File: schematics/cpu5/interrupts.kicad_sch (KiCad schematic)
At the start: 16 parts, among them U83 74LS08, U84 74LS32, U85 74LS32, U86 74LS04, U87 74LS02, U88 74LS02, U89 74LS08, U90 74LS32, U91 74LS541, U92 74LS32

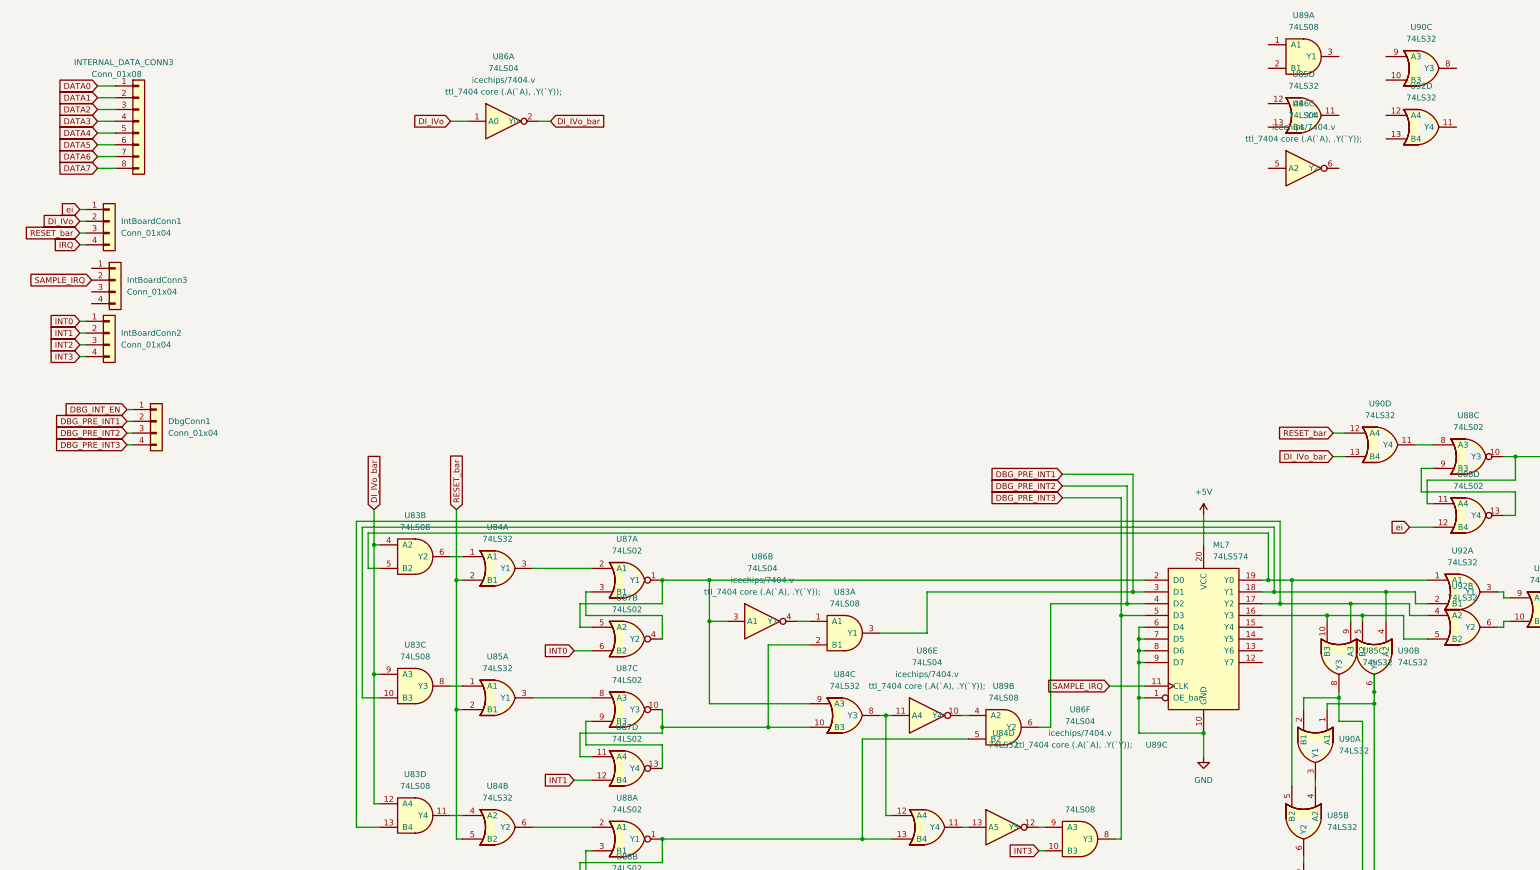
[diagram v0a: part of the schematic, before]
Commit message: start faults
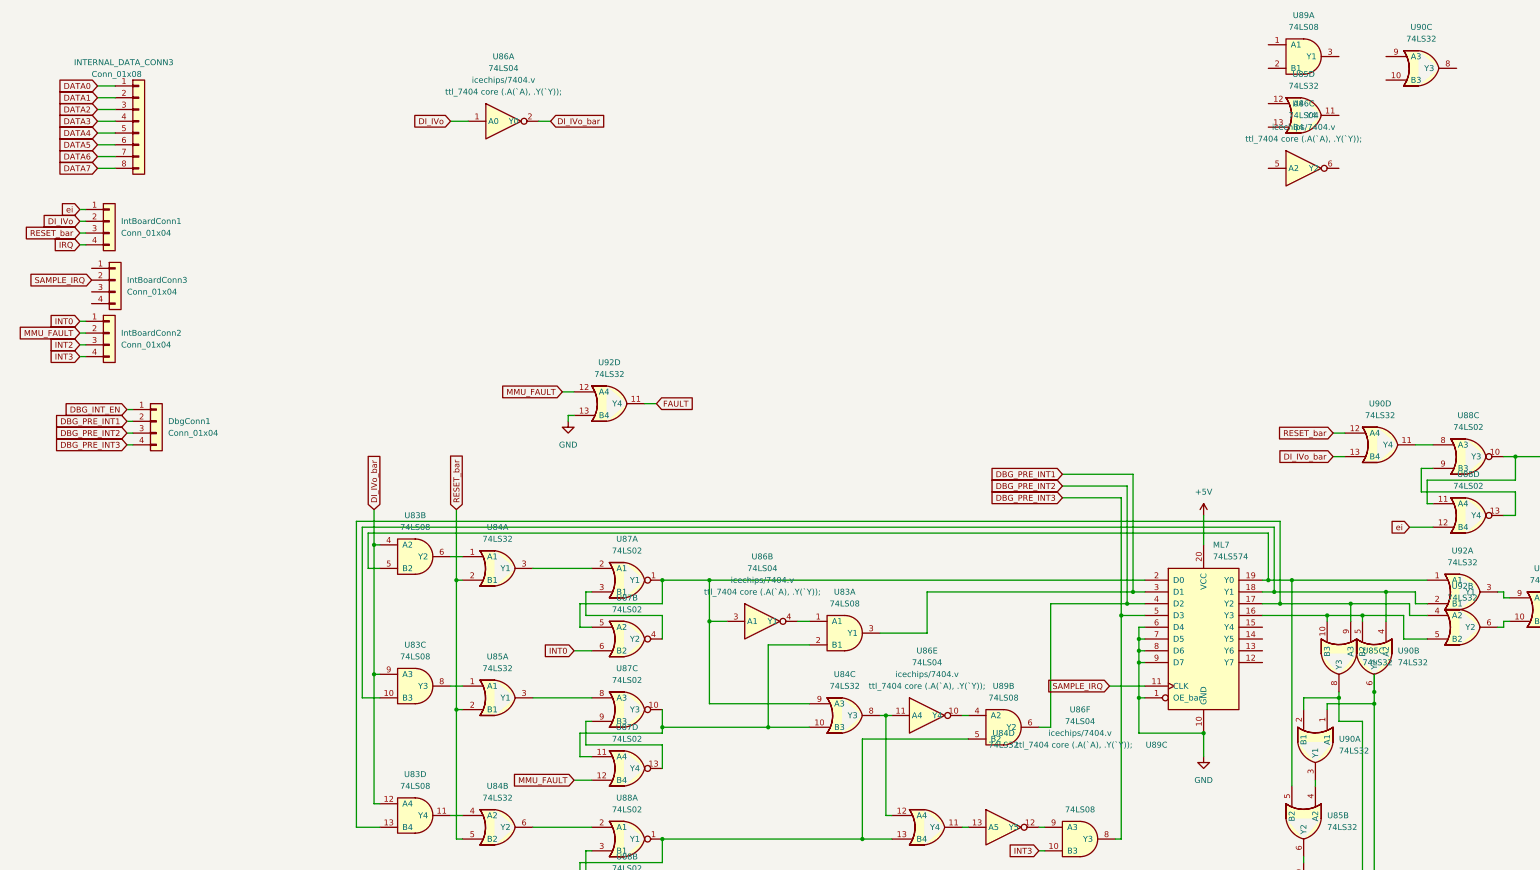
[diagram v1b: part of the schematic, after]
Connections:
- net INT1 is gone; now on net MMU_FAULT: IntBoardConn2.2 (Pin_2), U87.12 (B4)
- net GND: now also U92.13 (B4)
- net FAULT: now reaches U92.11 (Y4)
- net MMU_FAULT: now reaches U92.12 (A4)
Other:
- moved on the sheet: U92D

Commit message: faults seem to work
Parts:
- added U127: 74LS08, Package_DIP:DIP-14_W7.62mm, symbol 7400_ice:74LS08
- added U128, U129: 74LS74, Package_DIP:DIP-14_W7.62mm, symbol 7400_ice:74LS74
- added U130: 74LS04, Package_DIP:DIP-14_W7.62mm, symbol 7400_ice:74LS04
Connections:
- net INT3 is gone; now on net DBG_PRE_INT3: IntBoardConn2.4 (Pin_4), U89.10 (B3)
- net +5V: now also U127.14 (VCC), U128.10 (nS2), U128.12 (D2), U128.14 (VCC), U128.2 (D1), U128.4 (nS1), U129.14 (VCC), U129.2 (D1), U129.4 (nS1), U130.14 (VCC)
- net DBG_PRE_INT1: now also U83.2 (B1), U84.10 (B3), U128.9 (Q2); no longer ML7.3 (D1), U83.3 (Y1)
- net DBG_PRE_INT2: now also U84.13 (B4), U89.5 (B2), U129.5 (Q1); no longer ML7.4 (D2), U89.6 (Y2)
- net DBG_PRE_INT3: no longer ML7.5 (D3), U89.8 (Y3)
- net GND: now also U127.7 (GND), U128.7 (GND), U129.7 (GND), U130.7 (GND)
- net INT0: now also U128.3 (Clk1); no longer U87.6 (B2)
- net INT2: now also U129.3 (Clk1); no longer U88.6 (B2)
- net MMU_FAULT: now also U128.11 (Clk2); no longer U87.12 (B4)
- net at U85.3 (Y1): now also U130.3 (A1); no longer U87.8 (A3)
- net DBG_PRE_INT0: now reaches ML7.2 (D0), U84.9 (A3), U86.3 (A1)
- net DBG_PRE_INT0: now also U128.5 (Q1); no longer U87.1 (Y1), U87.5 (A2)
- net at U88.2 (A1): no longer U84.6 (Y2)
- net at U88.3 (B1): no longer U88.4 (Y2)
- net at U87.4 (Y2): no longer U87.3 (B1)
- net at U84.3 (Y1): now also U130.1 (A0); no longer U87.2 (A1)
- net at U87.9 (B3): no longer U87.13 (Y4)
- new net: U128.1 (nR1), U130.2 (Y0)
- new net: U129.1 (nR1), U130.6 (Y2)
- new net: ML7.3 (D1), U83.3 (Y1)
- new net: ML7.5 (D3), U89.8 (Y3)
- new net: U130.5 (A2), U84.6 (Y2)
- new net: U128.13 (nR2), U130.4 (Y1)
- new net: ML7.4 (D2), U89.6 (Y2)
- now unconnected: U87.10 (Y3), U87.11 (A4), U88.1 (Y1), U88.5 (A2)
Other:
- moved on the sheet: U83B, U83C, U83D, U84A, U84B, U85A, U87A, U87B, U87C, U87D, U88A, U88B
